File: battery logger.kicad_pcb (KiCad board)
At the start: 2 copper layers, 65 x 50 mm, 49 parts, among them CON501 BARREL_JACK, IC301 ATMEGA328-P, J501 Net_Tie, P201 CONN_01X02, P301 CONN_01X12, P302 CONN_02X03, P303 CONN_01X12, P304 CONN_01X05, P601 CONN_01X04, Q201 BUK9575, SW301 SW_PUSH, U201 TS922, U401 TLC2274, U501 LM2931ADT-5.0, U601 74HC14, X301 CRYSTAL 16MHZ

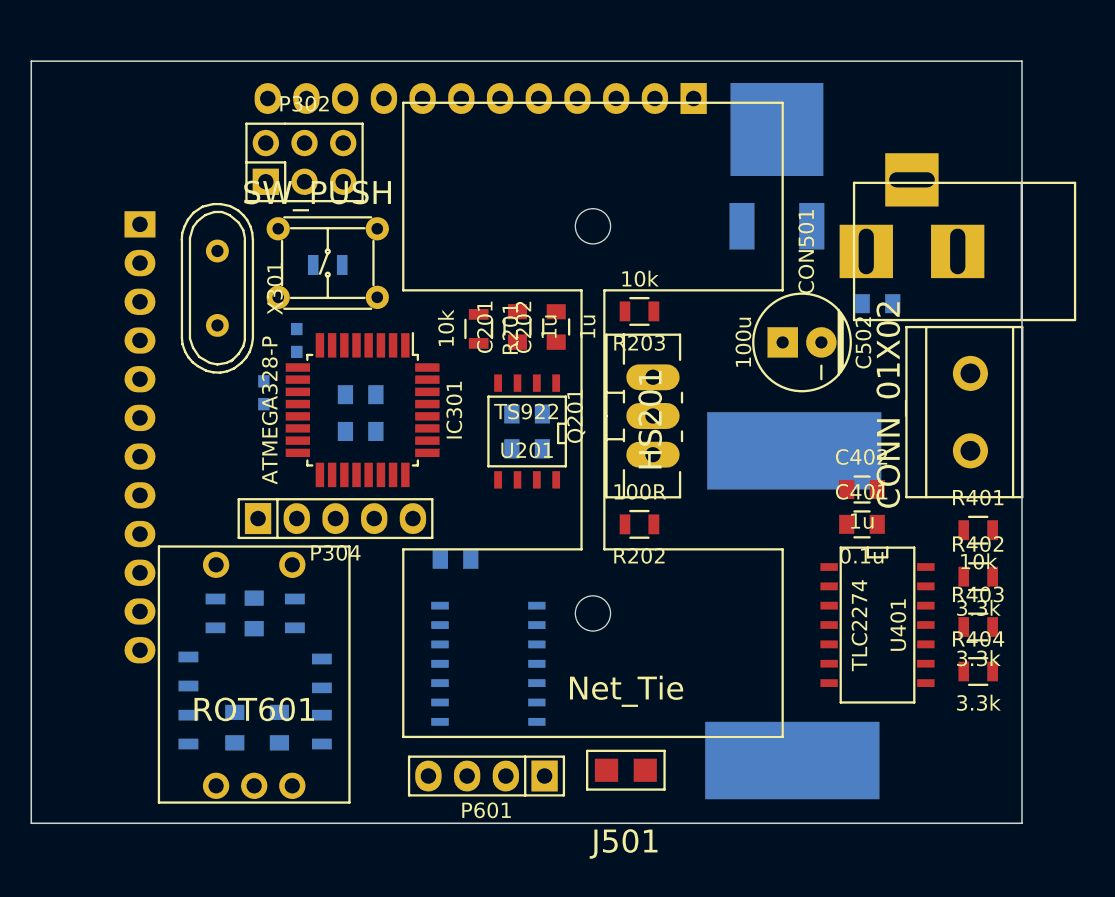
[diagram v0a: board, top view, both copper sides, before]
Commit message: tweaking part layout
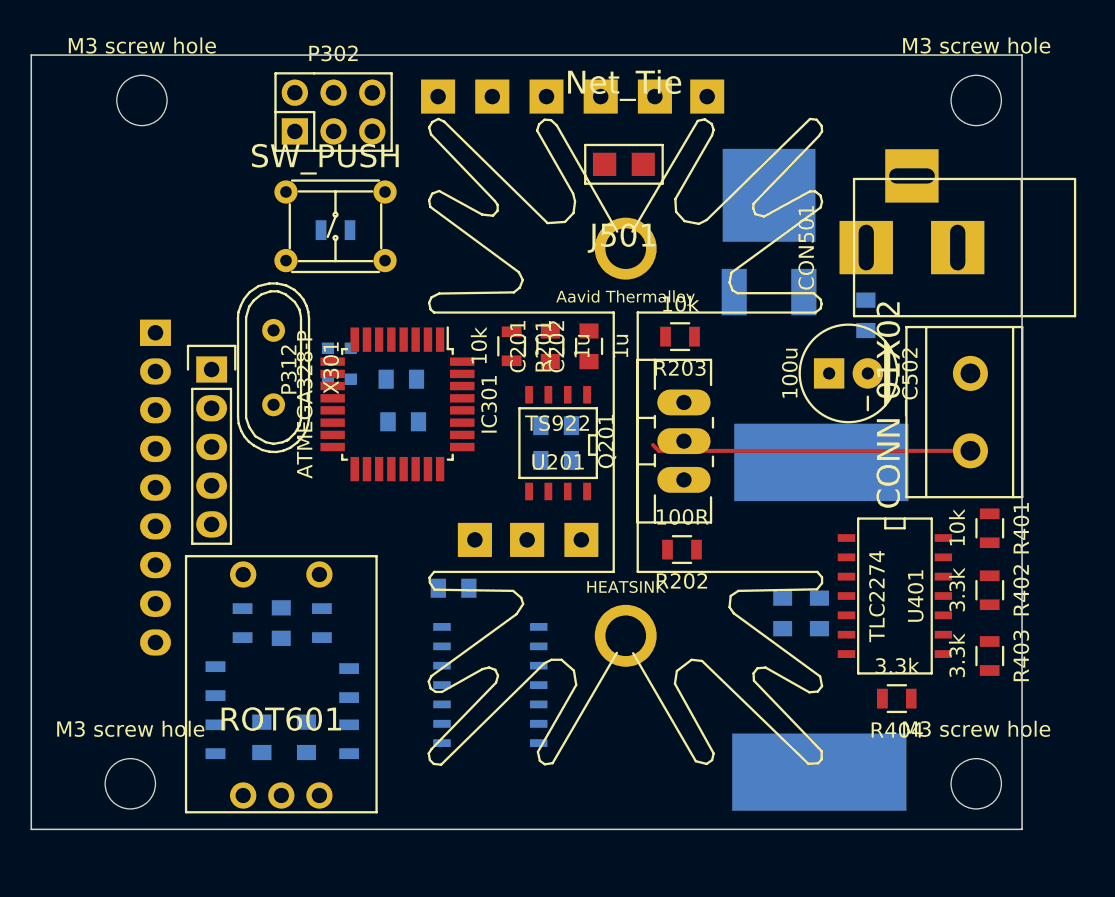
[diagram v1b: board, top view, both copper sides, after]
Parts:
- removed P601: CONN_01X04, Pin_Headers:Pin_Header_Straight_1x04
- added M3 screw hole: VAL**, battery logger:M3_screw_hole, F.Cu at (222.0, 52.6)
- added M3 screw hole: VAL**, battery logger:M3_screw_hole, F.Cu at (222.0, 97.4)
- added M3 screw hole: VAL**, battery logger:M3_screw_hole, F.Cu at (166.5, 97.4)
- added M3 screw hole: VAL**, battery logger:M3_screw_hole, F.Cu at (167.3, 52.6)
- added P305: CONN_01X01, Pin_Headers:Pin_Header_Straight_1x01, B.Cu at (197.4, 52.3)
- added P306: CONN_01X01, Pin_Headers:Pin_Header_Straight_1x01, B.Cu at (193.8, 52.3)
- added P307: CONN_01X01, Pin_Headers:Pin_Header_Straight_1x01, B.Cu at (190.2, 52.3)
- added P308: CONN_01X01, Pin_Headers:Pin_Header_Straight_1x01, B.Cu at (186.7, 52.3)
- added P309: CONN_01X01, Pin_Headers:Pin_Header_Straight_1x01, B.Cu at (189.1, 81.4)
- added P310: CONN_01X01, Pin_Headers:Pin_Header_Straight_1x01, B.Cu at (192.5, 81.4)
- added P311: CONN_01X01, Pin_Headers:Pin_Header_Straight_1x01, B.Cu at (196.1, 81.4)
- added P312: CONN_01X05, Socket_Strips:Socket_Strip_Straight_1x05, F.Cu at (171.8, 70.2)
- C401, C402: moved to B.Cu
- HS201: footprint battery logger:FA-T220-38E -> battery logger:FA-TO220-64E
- P301: value CONN_01X12 -> CONN_01X09; footprint Pin_Headers:Pin_Header_Straight_1x12 -> Pin_Headers:Pin_Header_Straight_1x09
- P303: value CONN_01X12 -> CONN_01X01; footprint Pin_Headers:Pin_Header_Straight_1x12 -> Pin_Headers:Pin_Header_Straight_1x01
- P304: value CONN_01X05 -> CONN_01X01; footprint Socket_Strips:Socket_Strip_Straight_1x05 -> Pin_Headers:Pin_Header_Straight_1x01; moved to B.Cu
- moved J501 39.8 mm to (198.9, 56.8)
- moved P304 34.7 mm to (200.9, 52.3), turned to 270 degrees
- moved P303 14.9 mm to (204.3, 52.3), turned to 90 degrees
- moved C402 9.65 mm to (209.3, 86.2), turned to 270 degrees
- moved P301 6.93 mm to (168.1, 67.8), turned to 180 degrees
- moved C401 6.48 mm to (211.7, 86.2), turned to 270 degrees
- moved X301 6.38 mm to (175.9, 70.1)
- moved R404 5.62 mm to (216.8, 91.8), turned to 180 degrees
- moved C302 5.03 mm to (180.2, 70.9), turned to 0 degrees
- moved U501 4.35 mm to (208.4, 65.2)
- moved P302 3.81 mm to (179.8, 53.3)
- moved C502 3.66 mm to (213.6, 70.5)
- moved R202 3.25 mm to (202.7, 82.0)
- moved R203 3.14 mm to (202.6, 68.1)
- moved C303 2.87 mm to (184.4, 73.7)
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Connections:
- P301 pad 4: /Encoder Interface/ENC_SW -> /uController/PD3
- P301 pad 5: /uController/PD3 -> /uController/PB6
- P301 pad 6: /Encoder Interface/ENC_A -> /uController/PB7
- P301 pad 7: /uController/PB6 -> /uController/PD6
- P301 pad 8: /uController/PB7 -> /uController/PD7
- P301 pad 9: /Encoder Interface/ENC_B -> /Current Sink/ENABLE
- P304 pad 1: /uController/LAT -> /Current Sink/I_SNS
- U601 pad 12: /Encoder Interface/ENC_SW -> /Encoder Interface/ENC_B
- U601 pad 13: Net-(C601-Pad1) -> Net-(C603-Pad1)
- U601 pad 8: /Encoder Interface/ENC_B -> /Encoder Interface/ENC_SW
- U601 pad 9: Net-(C603-Pad1) -> Net-(C601-Pad1)
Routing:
- net /Current Sink/BATT_V: track 0.00 -> 21.0 mm
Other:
- board size 65 x 50 mm -> 65 x 50.8 mm

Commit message: finished layout
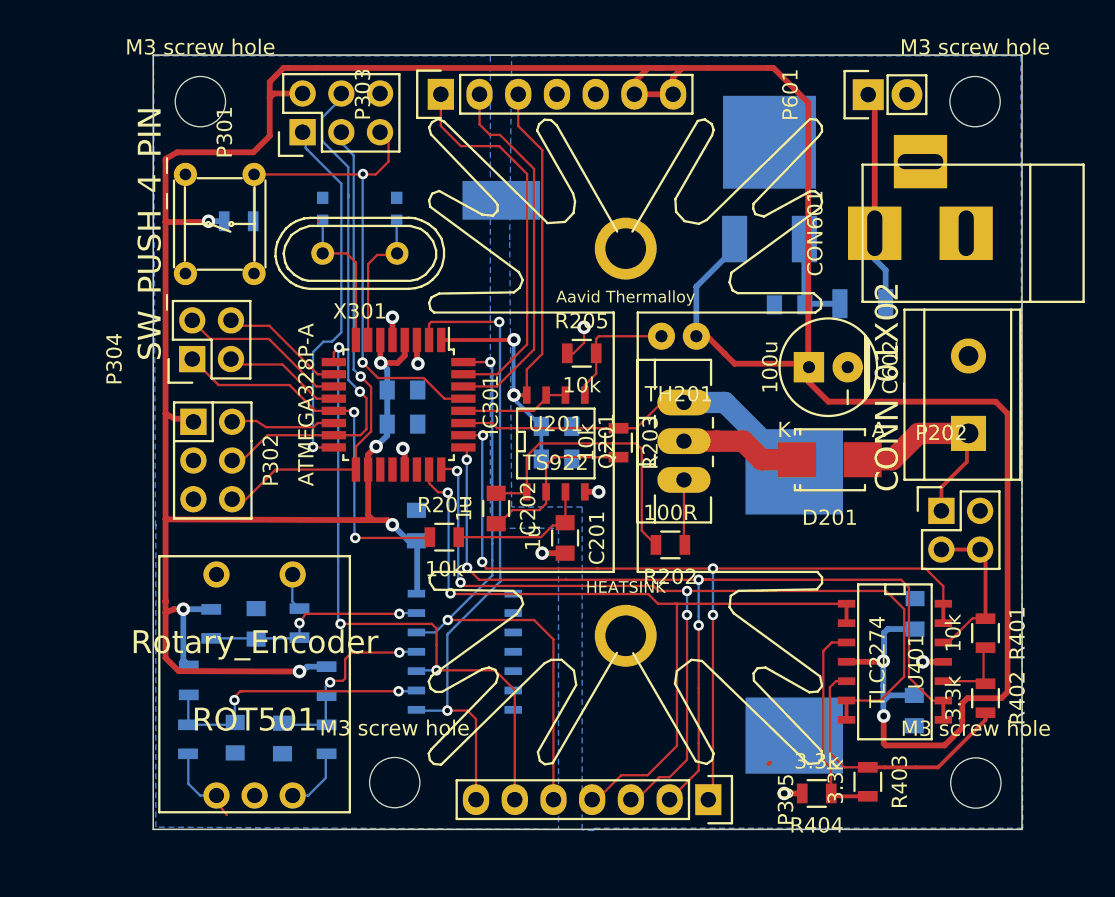
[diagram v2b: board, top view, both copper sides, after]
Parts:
- removed C603: 0.01u, Capacitors_SMD:C_0805
- removed C604: 0.1u, Capacitors_SMD:C_0805
- removed CON501: BARREL_JACK, Connect:BARREL_JACK
- removed J501: Net_Tie, battery logger:Net_Tie
- removed the M3 screw hole at (222.0, 52.6)
- removed the M3 screw hole at (222.0, 97.4)
- removed the M3 screw hole at (166.5, 97.4)
- removed the M3 screw hole at (167.3, 52.6)
- removed P306, P307, P308, P309, P310, P311: CONN_01X01, Pin_Headers:Pin_Header_Straight_1x01
- removed P312: CONN_01X05, Socket_Strips:Socket_Strip_Straight_1x05
- removed R601, R602, R603, R604, R605, R606: 10k, Resistors_SMD:R_0805
- removed ROT601: Rotary_Encoder, battery logger:PEC11R
- added C503: 0.01u, Capacitors_SMD:C_0805, B.Cu at (173.4, 94.4)
- added C504: 0.1u, Capacitors_SMD:C_0805, B.Cu at (185.3, 80.5)
- added CON601: BARREL_JACK, Connect:BARREL_JACK, F.Cu at (221.5, 61.3)
- added D201: DIODESCH, Diodes_SMD:Diode-SMB_Standard, F.Cu at (212.4, 76.1)
- added F601: FUSE, battery logger:PTC_1206, B.Cu at (214.6, 65.9)
- added J601: Net_Tie, battery logger:Net_Tie2, B.Cu at (190.8, 59.1)
- added M3 screw hole: VAL**, battery logger:M3_screw_hole, F.Cu at (222.0, 97.4)
- added M3 screw hole: VAL**, battery logger:M3_screw_hole, F.Cu at (183.8, 97.3)
- added M3 screw hole: VAL**, battery logger:M3_screw_hole, F.Cu at (171.1, 52.7)
- added M3 screw hole: VAL**, battery logger:M3_screw_hole, F.Cu at (221.9, 52.7)
- added P202: CONN_02X02, Pin_Headers:Pin_Header_Straight_2x02, F.Cu at (219.7, 79.5)
- added P601: CONN_01X02, Pin_Headers:Pin_Header_Straight_1x02, F.Cu at (214.9, 52.2)
- added R205: 10k, Resistors_SMD:R_0805, F.Cu at (196.1, 69.2)
- added R501: 10k, Resistors_SMD:R_0805, B.Cu at (177.6, 86.9)
- added R502: 10k, Resistors_SMD:R_0805, B.Cu at (171.8, 86.9)
- added R503: 10k, Resistors_SMD:R_0805, B.Cu at (179.4, 94.5)
- added R504: 10k, Resistors_SMD:R_0805, B.Cu at (179.4, 90.7)
- added R505: 10k, Resistors_SMD:R_0805, B.Cu at (170.3, 94.5)
- added R506: 10k, Resistors_SMD:R_0805, B.Cu at (170.3, 90.6)
- added ROT501: Rotary_Encoder, battery logger:PEC11R, F.Cu at (174.7, 90.7)
- added TH201: THERMISTOR, battery logger:SolderWirePad_2x_0-8mmDrill, F.Cu at (202.5, 68.0)
- C501: value 0.1u -> 1u
- C502: value 100u -> 0.01u; footprint battery logger:Capacitor6.4x6RM2.5 -> Capacitors_SMD:C_0805; moved to B.Cu
- C601: value 1u -> 0.1u
- C602: value 0.01u -> 100u; footprint Capacitors_SMD:C_0805 -> battery logger:Capacitor6.4x6RM2.5; moved to F.Cu
- IC301: value ATMEGA328-P -> ATMEGA328P-A
- P301: value CONN_01X09 -> CONN_02X03; footprint Pin_Headers:Pin_Header_Straight_1x09 -> Pin_Headers:Pin_Header_Straight_2x03; moved to F.Cu
- P303, P305: value CONN_01X01 -> CONN_01X07; footprint Pin_Headers:Pin_Header_Straight_1x01 -> Pin_Headers:Pin_Header_Straight_1x07; moved to F.Cu
- P304: value CONN_01X01 -> CONN_02X02; footprint Pin_Headers:Pin_Header_Straight_1x01 -> Pin_Headers:Pin_Header_Straight_2x02; moved to F.Cu
- R204: footprint battery logger:FA -> battery logger:8035_J-Lead
- SW301: value SW_PUSH -> SW_PUSH_4_PIN
- U501: value LM2931ADT-5.0 -> 74HC14; footprint SMD_Packages:DPAK-2 -> SMD_Packages:SOIC-14_N
- U601: value 74HC14 -> LM2931ADT-5.0; footprint SMD_Packages:SOIC-14_N -> SMD_Packages:DPAK-2
- moved P305 46.7 mm to (204.4, 98.5), turned to 270 degrees
- moved C501 44.8 mm to (174.8, 86.9), turned to 90 degrees
- moved C502 44.2 mm to (176.5, 94.4)
- moved C602 42.0 mm to (212.3, 70.1)
- moved C601 39.3 mm to (209.8, 66.0), turned to 180 degrees
- moved P304 34.9 mm to (170.6, 69.5), turned to 90 degrees
- moved U601 34.6 mm to (208.4, 61.7), turned to 180 degrees
- moved U501 31.0 mm to (188.3, 88.7), turned to 270 degrees
- moved P302 24.2 mm to (171.9, 76.2), turned to 270 degrees
- moved P303 17.5 mm to (186.9, 52.2)
- moved P301 16.3 mm to (177.8, 54.7), turned to 90 degrees
- moved R201 13.3 mm to (187.1, 81.2), turned to 0 degrees
- moved C201 12.6 mm to (195.0, 81.3), turned to 270 degrees
- moved C202 12.3 mm to (190.5, 79.3), turned to 270 degrees
- moved R403 11.5 mm to (214.9, 97.3)
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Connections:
- C201 pad 2: GND -> GNDD
- C501 pad 2: GND -> GNDD
- C502 pad 1: VCC -> Net-(C502-Pad1)
- C502 pad 2: GND -> GNDD
- C602 pad 1: Net-(C602-Pad1) -> VCC
- IC301 pad 1: /uController/PC6 -> /Current Sink/ENABLE
- IC301 pad 10: /uController/PB7 -> /uController/PD6
- IC301 pad 11: /Encoder Interface/ENC_B -> /uController/PD7
- IC301 pad 12: /uController/PD6 -> /uController/PB0
- IC301 pad 13: /uController/PD7 -> /Current Sink/V_SET
- IC301 pad 14: /Current Sink/ENABLE -> /uController/LAT
- IC301 pad 15: /Current Sink/V_SET -> /uController/DAT
- IC301 pad 16: /uController/LAT -> /uController/MISO
- IC301 pad 17: /uController/DAT -> /uController/CLK
- IC301 pad 18: /uController/PB4 -> VCC
- IC301 pad 19: /uController/CLK -> /uController/ADC6
- IC301 pad 2: /uController/PD0 -> /Encoder Interface/ENC_A
- IC301 pad 20: VCC -> /uController/AREF
- IC301 pad 21: /uController/AREF -> GNDD
- IC301 pad 22: GNDD -> /uController/ADC7
- IC301 pad 23: /Input Voltage Range Switch/V_SNS1 -> /Input Voltage Range Switch/V_SNS4
- IC301 pad 24: /Input Voltage Range Switch/V_SNS2 -> /Input Voltage Range Switch/V_SNS3
- IC301 pad 25: /Input Voltage Range Switch/V_SNS3 -> /Input Voltage Range Switch/V_SNS2
- IC301 pad 26: /Input Voltage Range Switch/V_SNS4 -> /Input Voltage Range Switch/V_SNS1
- IC301 pad 28: /uController/PC5 -> /Current Sink/AUX
- IC301 pad 29: (no net) -> /uController/PC6
- IC301 pad 3: /uController/PD1 -> GNDD
- IC301 pad 30: (no net) -> /uController/PD0
- IC301 pad 31: (no net) -> /uController/PD1
- IC301 pad 32: (no net) -> /Encoder Interface/ENC_SW
- IC301 pad 4: /Encoder Interface/ENC_SW -> VCC
- IC301 pad 5: /uController/PD3 -> GNDD
- IC301 pad 6: /Encoder Interface/ENC_A -> VCC
- IC301 pad 7: VCC -> /uController/PB6
- IC301 pad 8: GNDD -> /uController/PB7
- IC301 pad 9: /uController/PB6 -> /Encoder Interface/ENC_B
- P201 pad 1: /Current Sink/BATT_V -> Net-(D201-Pad1)
- P301 pad 1: /uController/PC6 -> /uController/MISO
- P301 pad 2: /uController/PD0 -> VCC
- P301 pad 3: /uController/PD1 -> /uController/CLK
- P301 pad 4: /uController/PD3 -> /uController/DAT
- P301 pad 5: /uController/PB6 -> /uController/PC6
- P301 pad 6: /uController/PB7 -> GNDD
- P302 pad 1: /uController/PB4 -> VCC
- P302 pad 2: VCC -> /uController/LAT
- P302 pad 3: /uController/CLK -> GNDD
- P302 pad 5: /uController/PC6 -> GNDD
- P302 pad 6: GNDD -> /uController/CLK
- P303 pad 1: /uController/PC5 -> /uController/PD1
- P304 pad 1: /Current Sink/I_SNS -> /Current Sink/V_SET
- P305 pad 1: /Input Voltage Range Switch/V_SNS4 -> /Input Voltage Range Switch/V_SNS1
- Q201 pad D: /Current Sink/BATT_V -> Net-(D201-Pad2)
- SW301 pad 1: GND -> /uController/PC6
- SW301 pad 2: /uController/PC6 -> GNDD
- SW301 pad 3: (no net) -> GNDD
- SW301 pad 4: (no net) -> /uController/PC6
- U201 pad 5: (no net) -> Net-(R205-Pad2)
- U201 pad 6: (no net) -> /Current Sink/AUX
- U201 pad 7: (no net) -> /Current Sink/AUX
- U401 pad 1: /Input Voltage Range Switch/V_SNS1 -> /Input Voltage Range Switch/V_SNS4
- U401 pad 10: Net-(R402-Pad2) -> Net-(R401-Pad2)
- U401 pad 12: Net-(R403-Pad2) -> /Current Sink/BATT_V
- U401 pad 13: /Input Voltage Range Switch/V_SNS4 -> /Input Voltage Range Switch/V_SNS1
- U401 pad 14: /Input Voltage Range Switch/V_SNS4 -> /Input Voltage Range Switch/V_SNS1
- U401 pad 2: /Input Voltage Range Switch/V_SNS1 -> /Input Voltage Range Switch/V_SNS4
- U401 pad 3: /Current Sink/BATT_V -> Net-(R403-Pad2)
- U401 pad 5: Net-(R401-Pad2) -> Net-(R402-Pad2)
- U401 pad 6: /Input Voltage Range Switch/V_SNS2 -> /Input Voltage Range Switch/V_SNS3
- U401 pad 7: /Input Voltage Range Switch/V_SNS2 -> /Input Voltage Range Switch/V_SNS3
- U401 pad 8: /Input Voltage Range Switch/V_SNS3 -> /Input Voltage Range Switch/V_SNS2
- U401 pad 9: /Input Voltage Range Switch/V_SNS3 -> /Input Voltage Range Switch/V_SNS2
- U501 pad 1: Net-(C501-Pad1) -> Net-(U501-Pad1)
- U501 pad 2: GND -> Net-(U501-Pad2)
- U501 pad 3: VCC -> Net-(U501-Pad3)
- U601 pad 1: Net-(U601-Pad1) -> Net-(C601-Pad1)
- U601 pad 2: Net-(U601-Pad2) -> GND
- U601 pad 3: Net-(U601-Pad3) -> VCC
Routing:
- net VCC: track 0.00 -> 241.8 mm, vias 0 -> 8
- net /Input Voltage Range Switch/V_SNS2: track 0.00 -> 64.6 mm, vias 0 -> 4
- net /Input Voltage Range Switch/V_SNS3: track 0.00 -> 64.5 mm, vias 0 -> 4
- net /Input Voltage Range Switch/V_SNS1: track 0.00 -> 58.5 mm, vias 0 -> 4
- net /Input Voltage Range Switch/V_SNS4: track 0.00 -> 52.7 mm, vias 0 -> 2
- net /Encoder Interface/ENC_B: track 0.00 -> 43.0 mm, vias 0 -> 3
- net /Encoder Interface/ENC_A: track 0.00 -> 42.0 mm, vias 0 -> 2
- net /uController/PC6: track 0.00 -> 40.8 mm, vias 0 -> 2
- net /Encoder Interface/ENC_SW: track 0.00 -> 40.5 mm, vias 0 -> 2
- net /Current Sink/ENABLE: track 0.00 -> 35.0 mm, vias 0 -> 2
- net /uController/DAT: track 0.00 -> 33.5 mm, vias 0 -> 1
- net /uController/CLK: track 0.00 -> 33.1 mm, vias 0 -> 1
- net /Current Sink/I_SNS: track 0.00 -> 26.0 mm
- net /uController/PD1: track 0.00 -> 25.2 mm
- net /Current Sink/V_SET: track 0.00 -> 24.6 mm, vias 0 -> 2
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- added copper zone on B.Cu, net GND
- added copper zone on B.Cu, net GNDD
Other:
- board size 65 x 50.8 mm -> 57 x 50.8 mm
- net class Analog Signal added: clearance 0.1524, trace_width 0.1524, via_dia 0.6858, via_drill 0.3302
- net class Digital Signal added: clearance 0.1524, trace_width 0.1524, via_dia 0.6858, via_drill 0.3302
- net class Power added: clearance 0.254, trace_width 0.381, via_dia 0.889, via_drill 0.635
- rule trace_min: 0.254 -> 0.1524
- rule via_min_drill: 0.508 -> 0.3302
- rule via_min_size: 0.889 -> 0.6858
